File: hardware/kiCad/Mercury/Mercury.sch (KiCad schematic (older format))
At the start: 13 parts

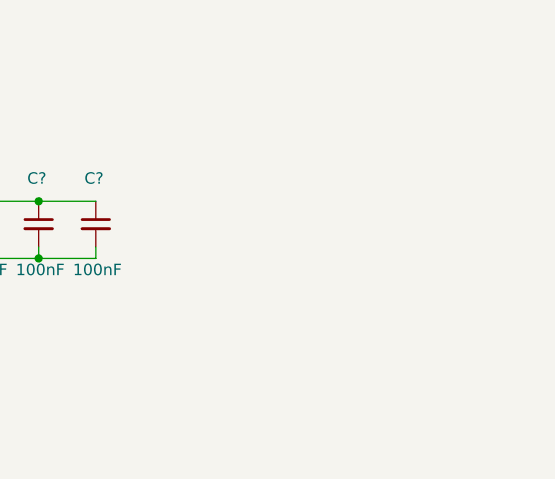
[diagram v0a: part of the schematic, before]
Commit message: VDDA
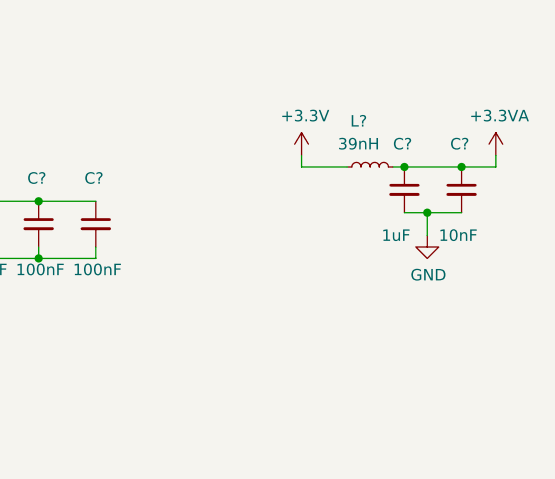
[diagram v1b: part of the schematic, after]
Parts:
- added C?: 1uF, symbol Device:C_Small
- added C?: 10nF, symbol Device:C_Small
- added L?: 39nH, symbol Device:L_Small
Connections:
- net +3.3VA: now also C?.1, C?.1, L?.2
- net +3V3: now also L?.1
- net GND: now also C?.2, C?.2
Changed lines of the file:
@@
 $EndComp
 Connection ~ 1900 1550
+$Comp
+L Device:L_Small L?
+U 1 1 5FE2984C
+P 5050 1150
+F 0 "L?" V 5250 1200 50  0000 C CNN
+F 1 "39nH" V 5150 1200 50  0000 C CNN
+F 2 "" H 5050 1150 50  0001 C CNN
+F 3 "~" H 5050 1150 50  0001 C CNN
+	1    5050 1150
+	0    -1   -1   0
+$EndComp
+$Comp
+L power:+3.3V #PWR?
+U 1 1 5FE29DC7
+P 4750 1100
+F 0 "#PWR?" H 4750 950 50  0001 C CNN
+F 1 "+3.3V" H 4765 1273 50  0000 C CNN
+F 2 "" H 4750 1100 50  0001 C CNN
+F 3 "" H 4750 1100 50  0001 C CNN
+	1    4750 1100
+	1    0    0    -1
+$EndComp
+Wire Wire Line
+	4750 1100 4750 1150
+Wire Wire Line
+	4750 1150 4950 1150
+$Comp
+L Device:C_Small C?
+U 1 1 5FE2B6A9
+P 5200 1250
+F 0 "C?" H 5150 1450 50  0000 L CNN
+F 1 "1uF" H 5100 1050 50  0000 L CNN
+F 2 "" H 5200 1250 50  0001 C CNN
+F 3 "~" H 5200 1250 50  0001 C CNN
+	1    5200 1250
+	1    0    0    -1
+$EndComp
+$Comp
+L Device:C_Small C?
+U 1 1 5FE2BF87
+P 5450 1250
+F 0 "C?" H 5400 1450 50  0000 L CNN
+F 1 "10nF" H 5350 1050 50  0000 L CNN
+F 2 "" H 5450 1250 50  0001 C CNN
+F 3 "~" H 5450 1250 50  0001 C CNN
+	1    5450 1250
+	1    0    0    -1
+$EndComp
+Wire Wire Line
+	5150 1150 5200 1150
+Wire Wire Line
+	5200 1150 5450 1150
+Connection ~ 5200 1150
+Wire Wire Line
+	5200 1350 5300 1350
+$Comp
+L power:+3.3VA #PWR?
+U 1 1 5FE3082E
+P 5600 1100
+F 0 "#PWR?" H 5600 950 50  0001 C CNN
+F 1 "+3.3VA" H 5615 1273 50  0000 C CNN
+F 2 "" H 5600 1100 50  0001 C CNN
+F 3 "" H 5600 1100 50  0001 C CNN
+	1    5600 1100
+	1    0    0    -1
+$EndComp
+Wire Wire Line
+	5450 1150 5600 1150
+Wire Wire Line
+	5600 1150 5600 1100
+Connection ~ 5450 1150
+$Comp
+L power:GND #PWR?
+U 1 1 5FE32675
+P 5300 1450
+F 0 "#PWR?" H 5300 1200 50  0001 C CNN
+F 1 "GND" H 5305 1277 50  0000 C CNN
+F 2 "" H 5300 1450 50  0001 C CNN
+F 3 "" H 5300 1450 50  0001 C CNN
+	1    5300 1450
+	1    0    0    -1
+$EndComp
+Wire Wire Line
+	5300 1450 5300 1350
+Connection ~ 5300 1350
+Wire Wire Line
+	5300 1350 5450 1350
 $EndSCHEMATC

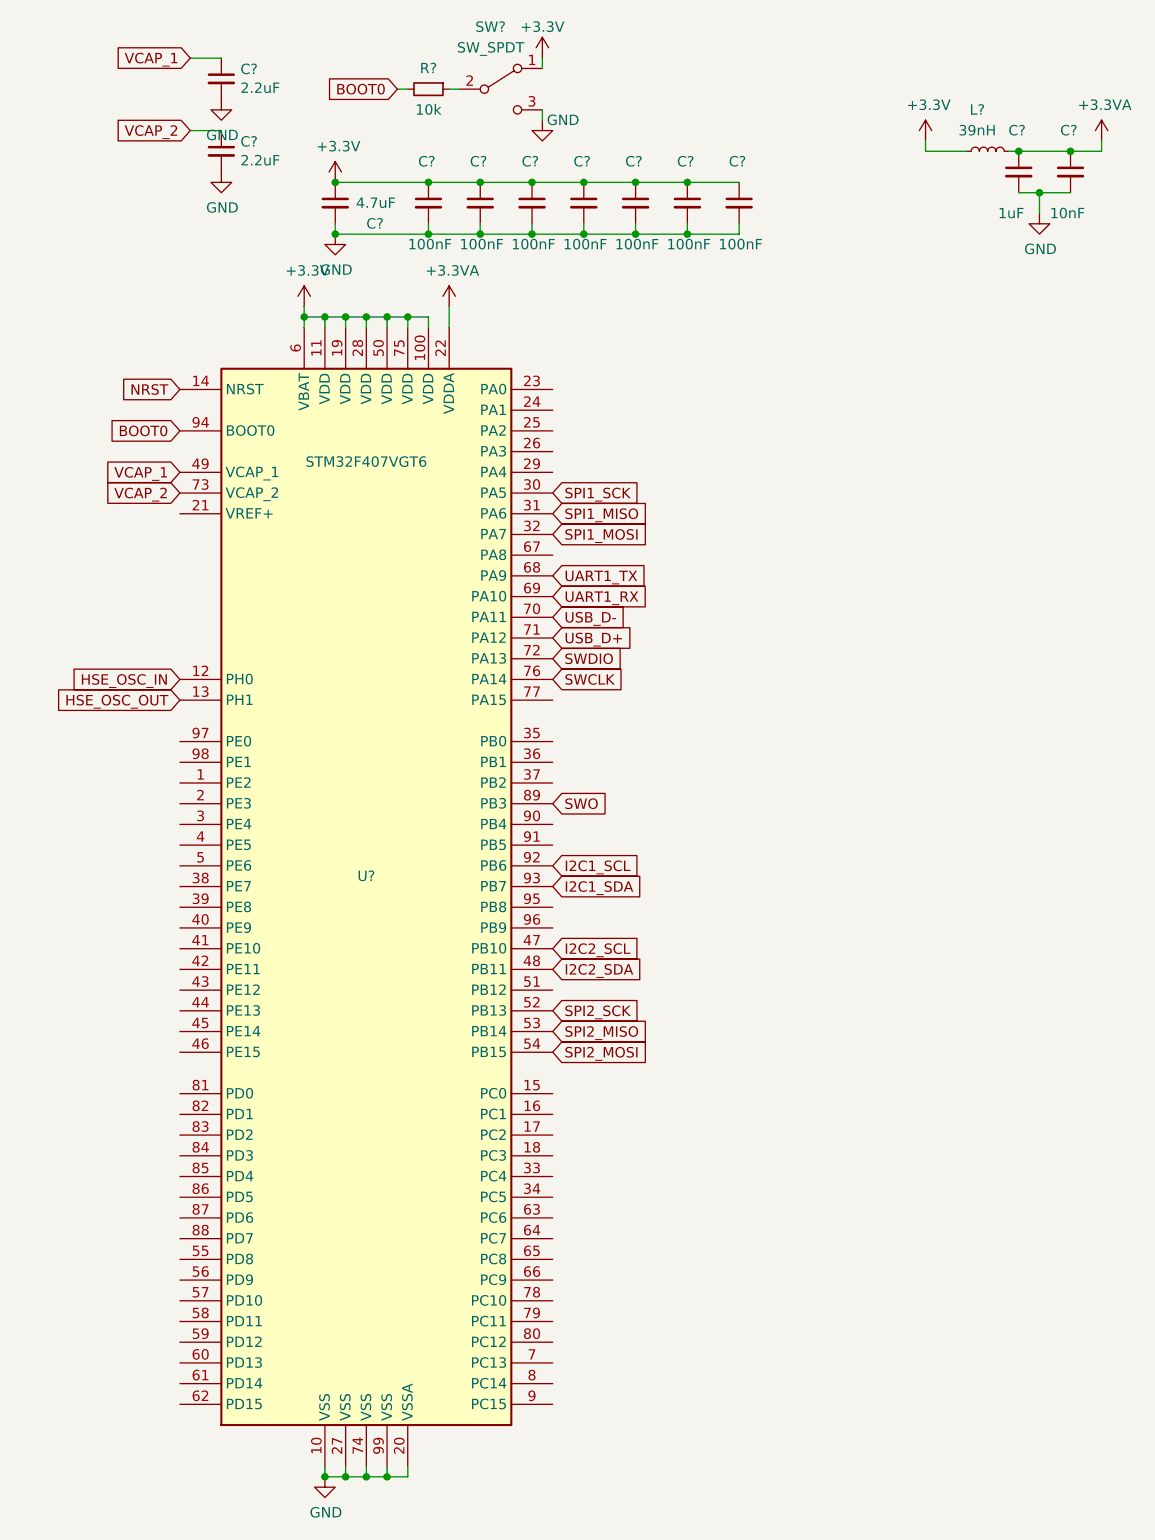
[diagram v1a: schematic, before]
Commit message: Clock
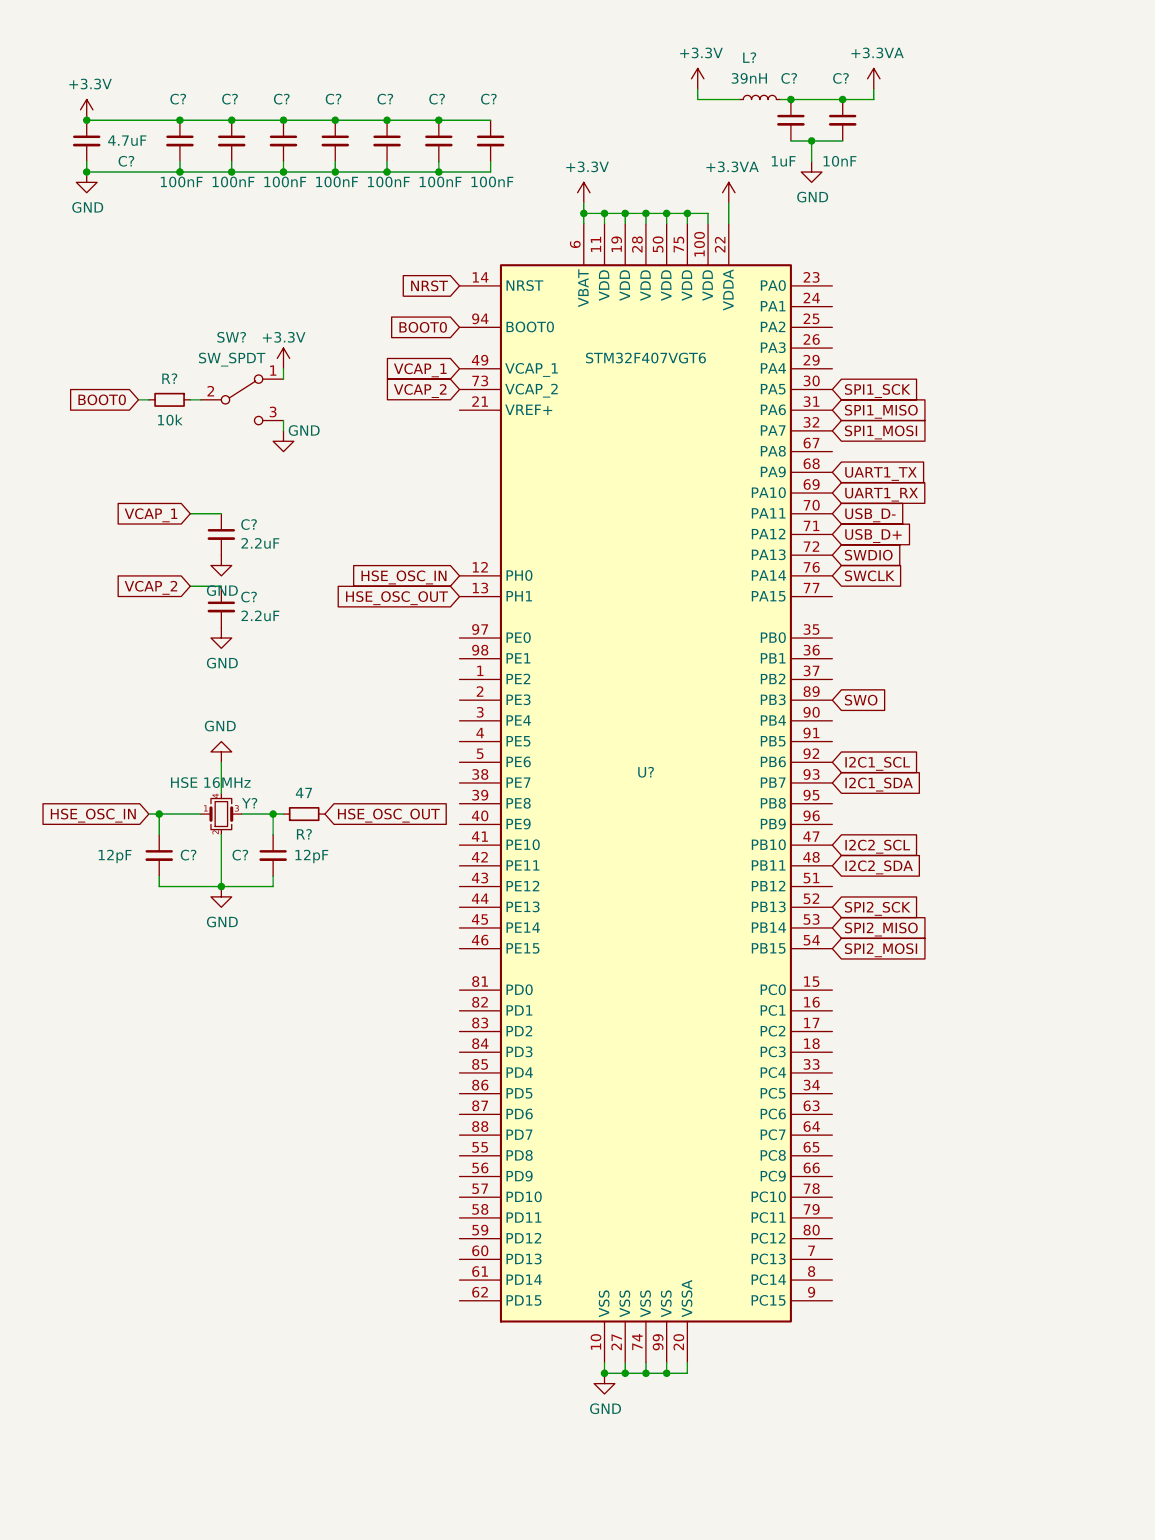
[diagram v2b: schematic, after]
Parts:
- added C? (x2): 12pF, symbol Device:C_Small
- added R?: 47, symbol Device:R_Small
- added Y?: HSE 16MHz, symbol Device:Crystal_GND24_Small
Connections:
- net GND: now also C?.2, C?.2, Y?.2, Y?.4
- net HSE_OSC_IN: now also C?.1, Y?.1
- net HSE_OSC_OUT: now also R?.2
- new net: C?.1, R?.1, Y?.3
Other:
- moved on the sheet: C?, L?, R?, SW?, U?
